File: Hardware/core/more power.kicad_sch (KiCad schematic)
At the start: 1 part

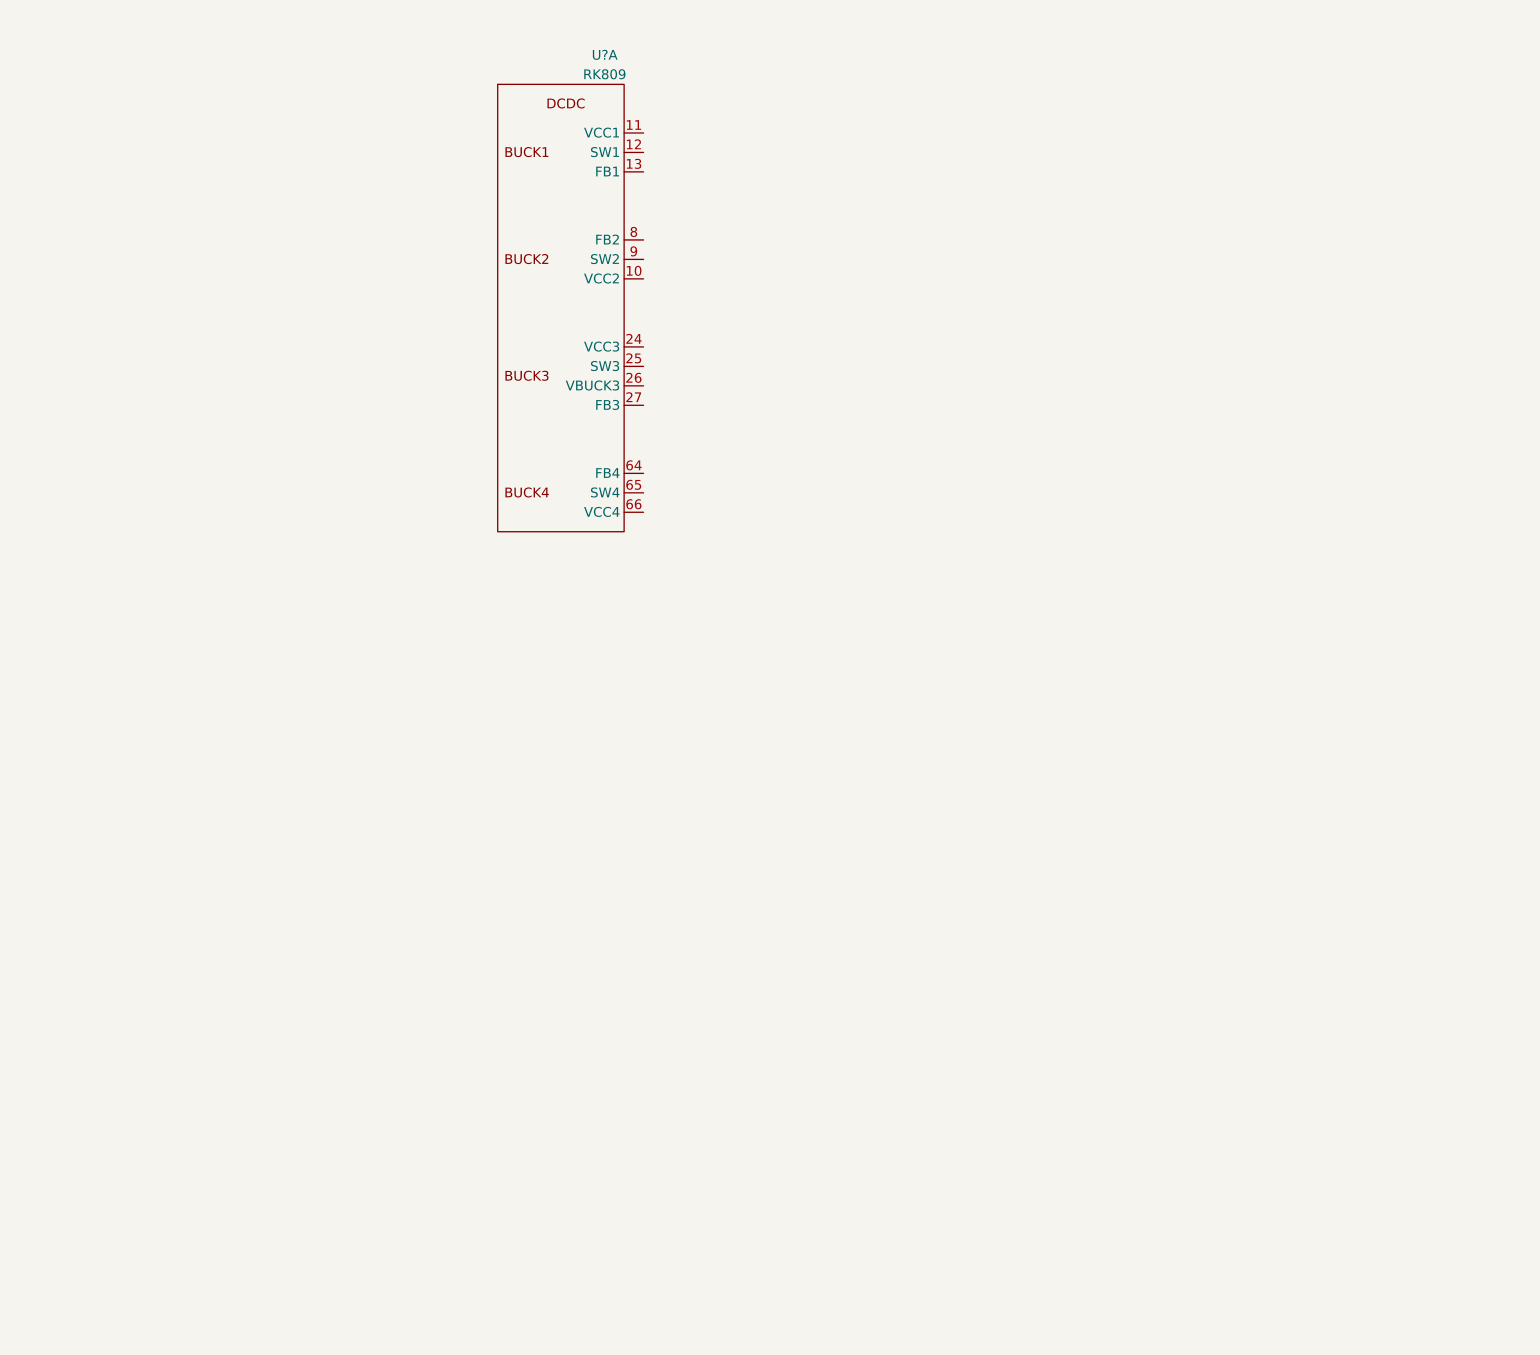
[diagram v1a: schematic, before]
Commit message: moooaaarr power
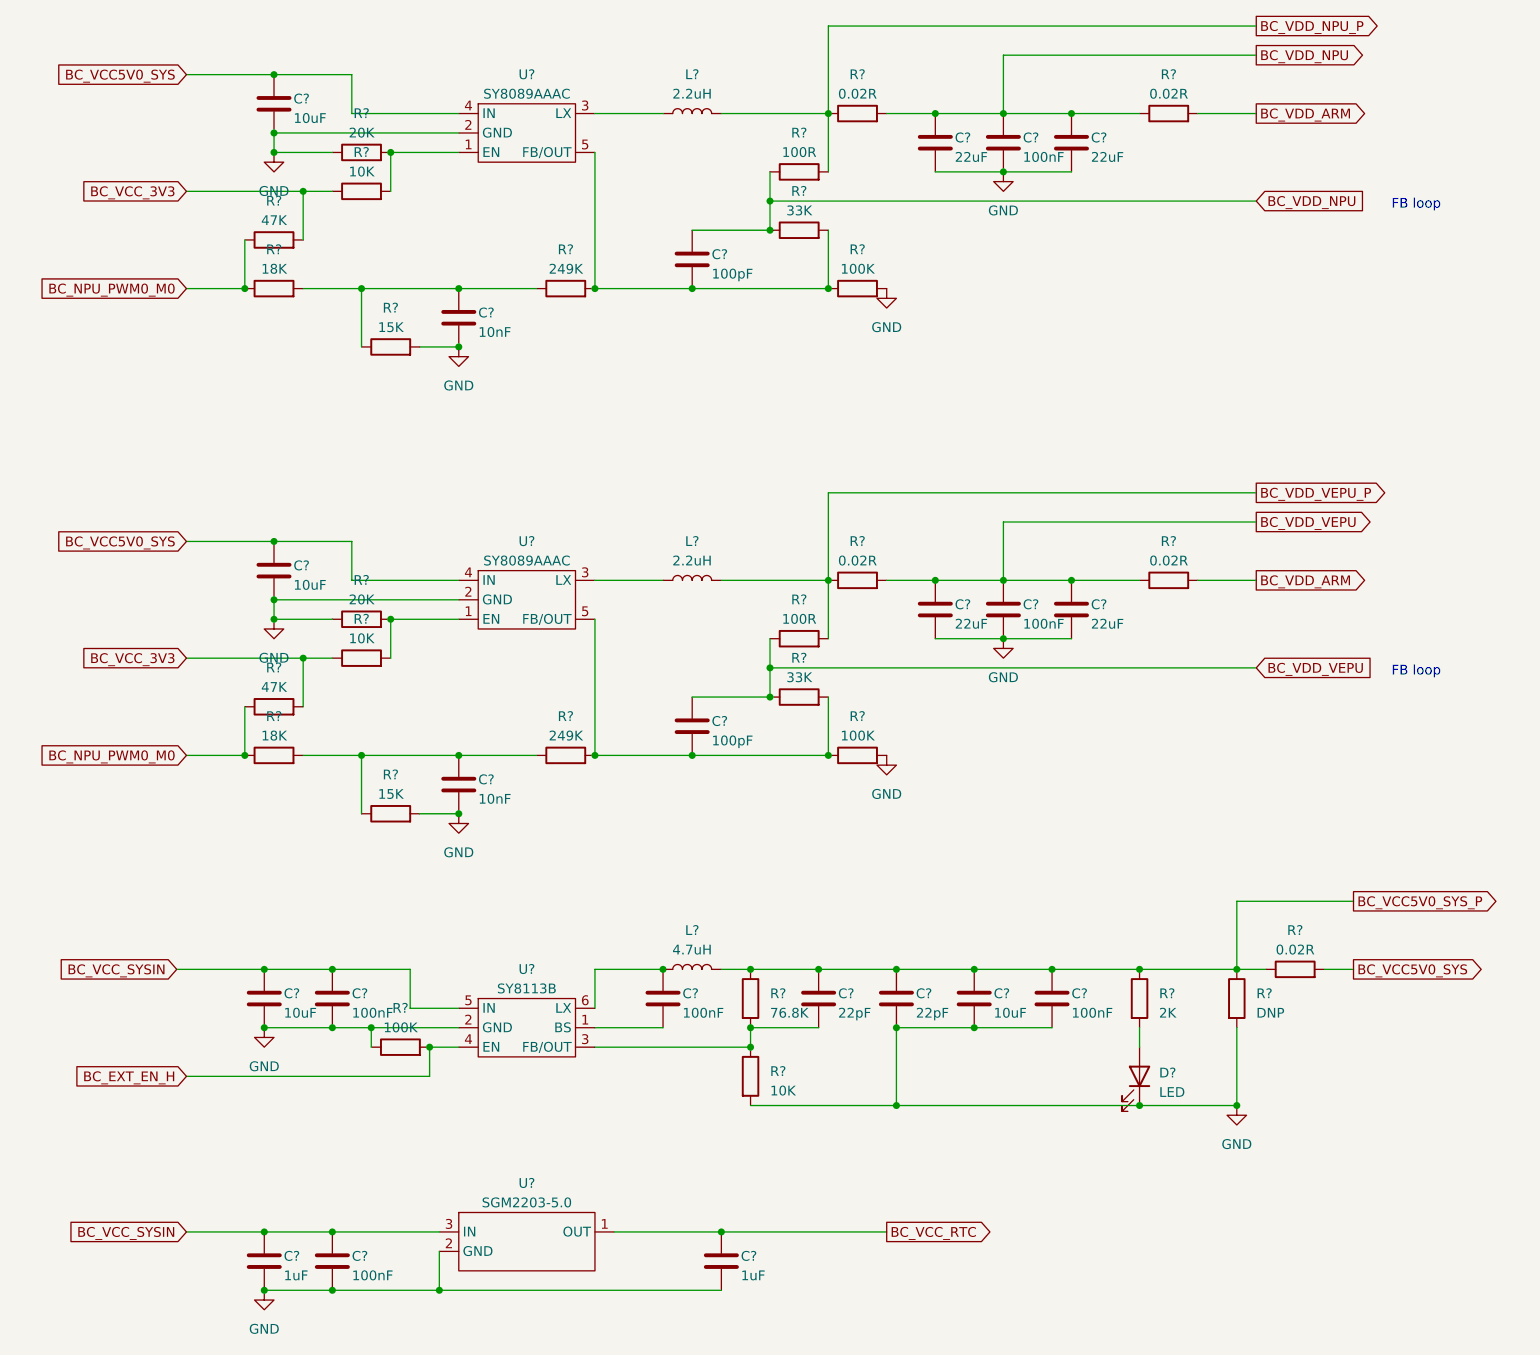
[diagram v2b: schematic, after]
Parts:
- removed U?: RK809, berryflight:QFN-68_EP_7x7_Pitch0.35mm, symbol berryflight:RK809
- added C? (x6): 100nF, Capacitor_SMD:C_0402_1005Metric, symbol Device:C
- added C? (x2): 1uF, Capacitor_SMD:C_0402_1005Metric, symbol Device:C
- added C? (x2): 10nF, Capacitor_SMD:C_0402_1005Metric, symbol Device:C
- added C? (x4): 22uF, Capacitor_SMD:C_0603_1608Metric, symbol Device:C
- added C?: 22pF, Capacitor_SMD:C_0402_1005Metric, symbol Device:C
- added C? (x4): 10uF, Capacitor_SMD:C_0805_2012Metric, symbol Device:C
- added C? (x2): 100pF, Capacitor_SMD:C_0402_1005Metric, symbol Device:C
- added C?: 22pF, Capacitor_SMD:C_0805_2012Metric, symbol Device:C
- added D?: LED, LED_SMD:LED_0603_1608Metric, symbol Device:LED
- added L? (x2): 2.2uH, Inductor_SMD:L_1008_2520Metric, symbol Device:L
- added L?: 4.7uH, Inductor_SMD:L_TracoPower_TCK-047_5.2x5.8mm, symbol Device:L
- added R? (x2): 18K, Resistor_SMD:R_0402_1005Metric, symbol Device:R
- added R?: 2K, Resistor_SMD:R_0402_1005Metric, symbol Device:R
- added R? (x2): 20K, Resistor_SMD:R_0402_1005Metric, symbol Device:R
- added R? (x5): 0.02R, Resistor_SMD:R_0805_2012Metric, symbol Device:R
- added R? (x3): 10K, Resistor_SMD:R_0402_1005Metric, symbol Device:R
- added R? (x3): 100K, Resistor_SMD:R_0402_1005Metric, symbol Device:R
- added R? (x2): 15K, Resistor_SMD:R_0402_1005Metric, symbol Device:R
- added R? (x2): 47K, Resistor_SMD:R_0402_1005Metric, symbol Device:R
- added R? (x2): 100R, Resistor_SMD:R_0402_1005Metric, symbol Device:R
- added R?: DNP, Resistor_SMD:R_0402_1005Metric, symbol Device:R
- added R? (x2): 33K, Resistor_SMD:R_0402_1005Metric, symbol Device:R
- added R? (x2): 249K, Resistor_SMD:R_0402_1005Metric, symbol Device:R
- added R?: 76.8K, Resistor_SMD:R_0402_1005Metric, symbol Device:R
- added U? (x2): SY8089AAAC, symbol berryflight:SY8089AAAC
- added U?: SGM2203-5.0, symbol berryflight:SGM2203-5.0
- added U?: SY8113B, symbol berryflight:SY8113B
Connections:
- new net: C?.1, L?.1, U?.6 (LX)
- new net: C?.2, U?.1 (BS)
- new net: C?.1, R?.1, R?.1, R?.2 (x2)
- new net: D?.2 (A), R?.2
- new net: R?.2, R?.2, U?.1 (EN) (x2)
- new net: L?.1, U?.3 (LX) (x2)
- new net: C?.2, R?.1, R?.2, R?.2, U?.5 (FB/OUT) (x2)
- new net: C?.2, R?.1, R?.2, U?.3 (FB/OUT)
- new net BC_EXT_EN_H: R?.2, U?.4 (EN)
- new net BC_NPU_PWM0_M0: R?.1, R?.1, R?.1, R?.1
- new net BC_VCC5V0_SYS: C?.1, C?.1, R?.2, U?.4 (IN), U?.4 (IN)
- new net BC_VCC5V0_SYS_P: C?.1, C?.1, C?.1, C?.1, L?.2, R?.1, R?.1, R?.1, R?.1
- new net BC_VCC_3V3: R?.1, R?.1, R?.2, R?.2
- new net BC_VCC_RTC: C?.1, U?.1 (OUT)
- new net BC_VCC_SYSIN: C?.1, C?.1, C?.1, C?.1, U?.3 (IN), U?.5 (IN)
- new net BC_VDD_ARM: R?.2, R?.2
- new net BC_VDD_NPU: C?.1, C?.1, C?.1, C?.1, R?.1, R?.1, R?.1, R?.2
- new net BC_VDD_NPU_P: L?.2, R?.1, R?.2
- new net BC_VDD_VEPU: C?.1, C?.1, C?.1, C?.1, R?.1, R?.1, R?.1, R?.2
- new net BC_VDD_VEPU_P: L?.2, R?.1, R?.2
- new net GND: C?.2, C?.2, C?.2, C?.2, C?.2, C?.2, C?.2, C?.2, C?.2, C?.2, C?.2, C?.2, C?.2, C?.2, C?.2, C?.2, C?.2, C?.2, D?.1 (K), R?.1, R?.1, R?.1, R?.2, R?.2, R?.2, R?.2, R?.2, R?.2, U?.2 (GND), U?.2 (GND), U?.2 (GND), U?.2 (GND)
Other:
- note added: "FB loop"
